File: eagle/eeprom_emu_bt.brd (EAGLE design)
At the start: 100 x 80 mm, 10 parts

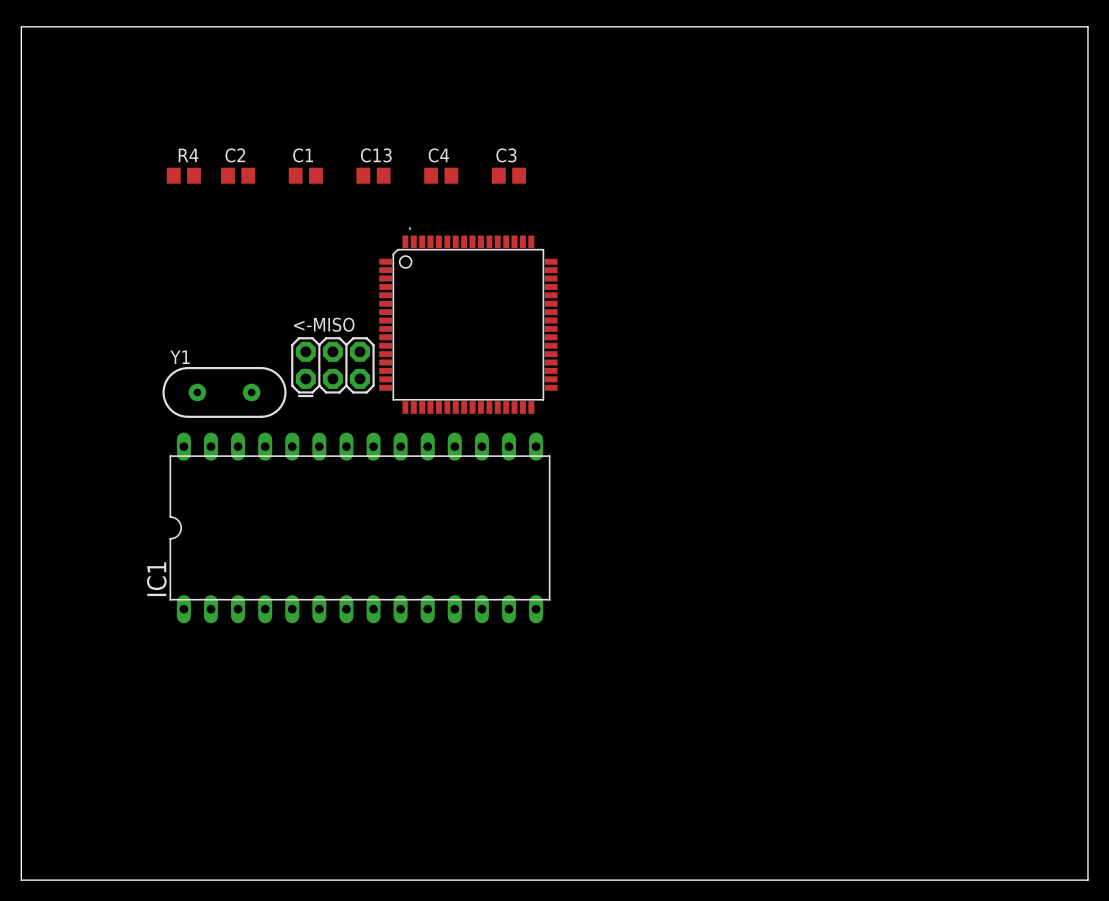
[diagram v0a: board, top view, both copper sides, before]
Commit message: eagles
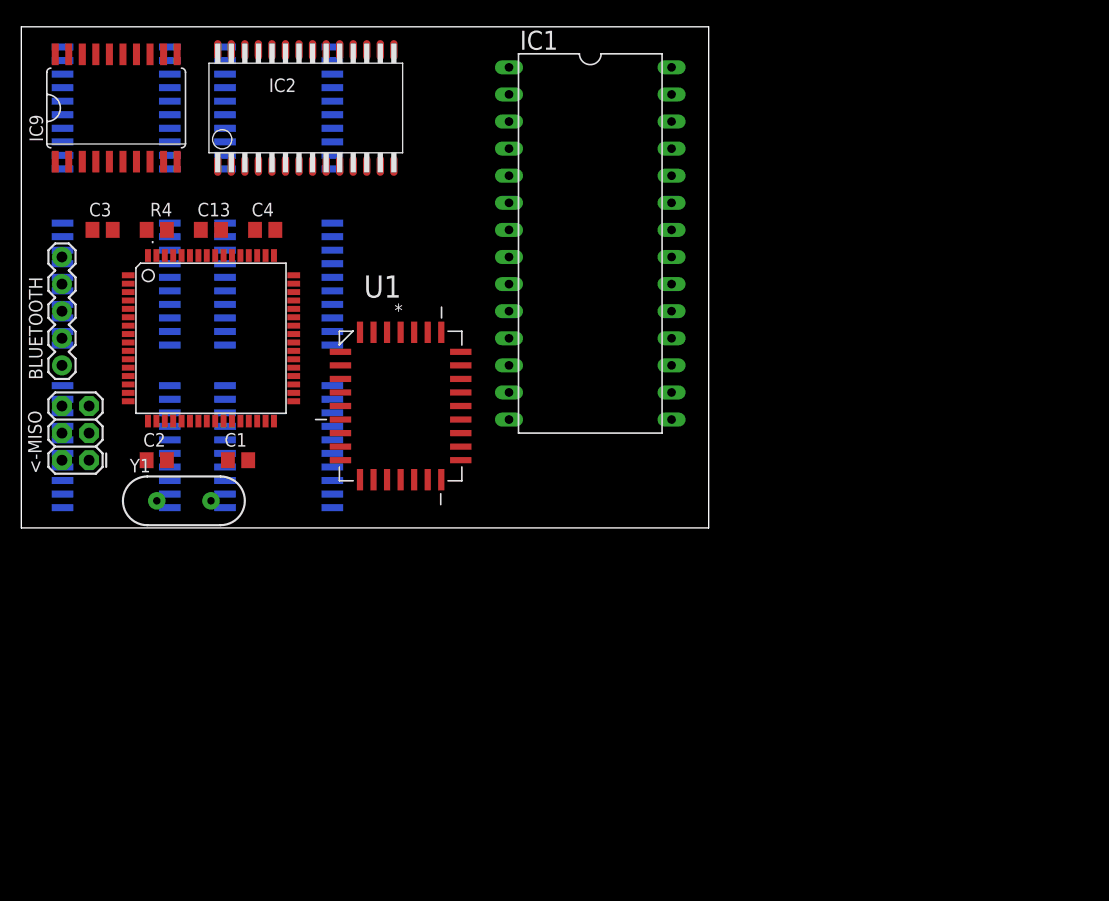
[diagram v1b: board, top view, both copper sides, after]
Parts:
- added BLUETOOTH: (no value), SparkFun-Connectors:1X05
- added IC2: IS62C256AL-45U, memory-issi-asynsram:SOP28-330MIL
- added IC3, IC4, IC5, IC6, IC7, IC8: 74HCT541DW, 74xx-eu:SO20W
- added IC9: 74HC573D, 74xx-eu:SO20W
- added U1: SST39SF040-70-4I-NHE, Silicon_Storage_Tech_By_element14_Batch_1:PLCC127P1244X1498X357-32N
- moved C3 38.4 mm to (7.62, 61.0)
- moved IC1 34.3 mm to (53.3, 59.7), turned to 270 degrees
- moved C2 27.7 mm to (12.7, 39.4)
- moved C1 27.4 mm to (20.3, 39.4)
- moved . 24.2 mm to (17.8, 50.8)
- moved <-MISO 21.7 mm to (6.35, 39.4), turned to 90 degrees
- moved C4 17.3 mm to (22.9, 61.0)
- moved C13 16.1 mm to (17.8, 61.0)
- moved Y1 10.9 mm to (15.2, 35.6)
- moved R4 5.68 mm to (12.7, 61.0)
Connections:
- new net VDD: IC2.28, U1.32
- net GND: now also IC2.14, IC3.10, IC4.10, IC5.10, IC6.10, IC7.10, IC8.10, IC9.10
- net VCC: now also IC3.20, IC4.20, IC5.20, IC6.20, IC7.20, IC8.20, IC9.20
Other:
- board size 100 x 80 mm -> 64.4 x 47 mm
